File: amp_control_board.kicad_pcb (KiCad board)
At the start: 2 copper layers, 75 parts, among them J1 Conn_01x03_Male, J2 Conn_01x04_Female, J3 Screw_Terminal_01x03, J4 Screw_Terminal_01x02, J5 Conn_01x04_Female, J6 Conn_02x03_Odd_Even, J7 Conn_01x03_Male, M1 Fan_4pin, M2 Fan_4pin, Q1 BSP89, Q2 BSP89, Q3 BSS138, Q4 BSS138, SW1 SW_Push, SW2 SW_Push, SW3 SW_Push, SW4 SW_Push, U1 L7805, U2 L7812, U3 LD1117V33-DG, U4 MCP4251-xxxx-SL, U5 STM32F103C8Tx, Y1 8M, Y2 32.768

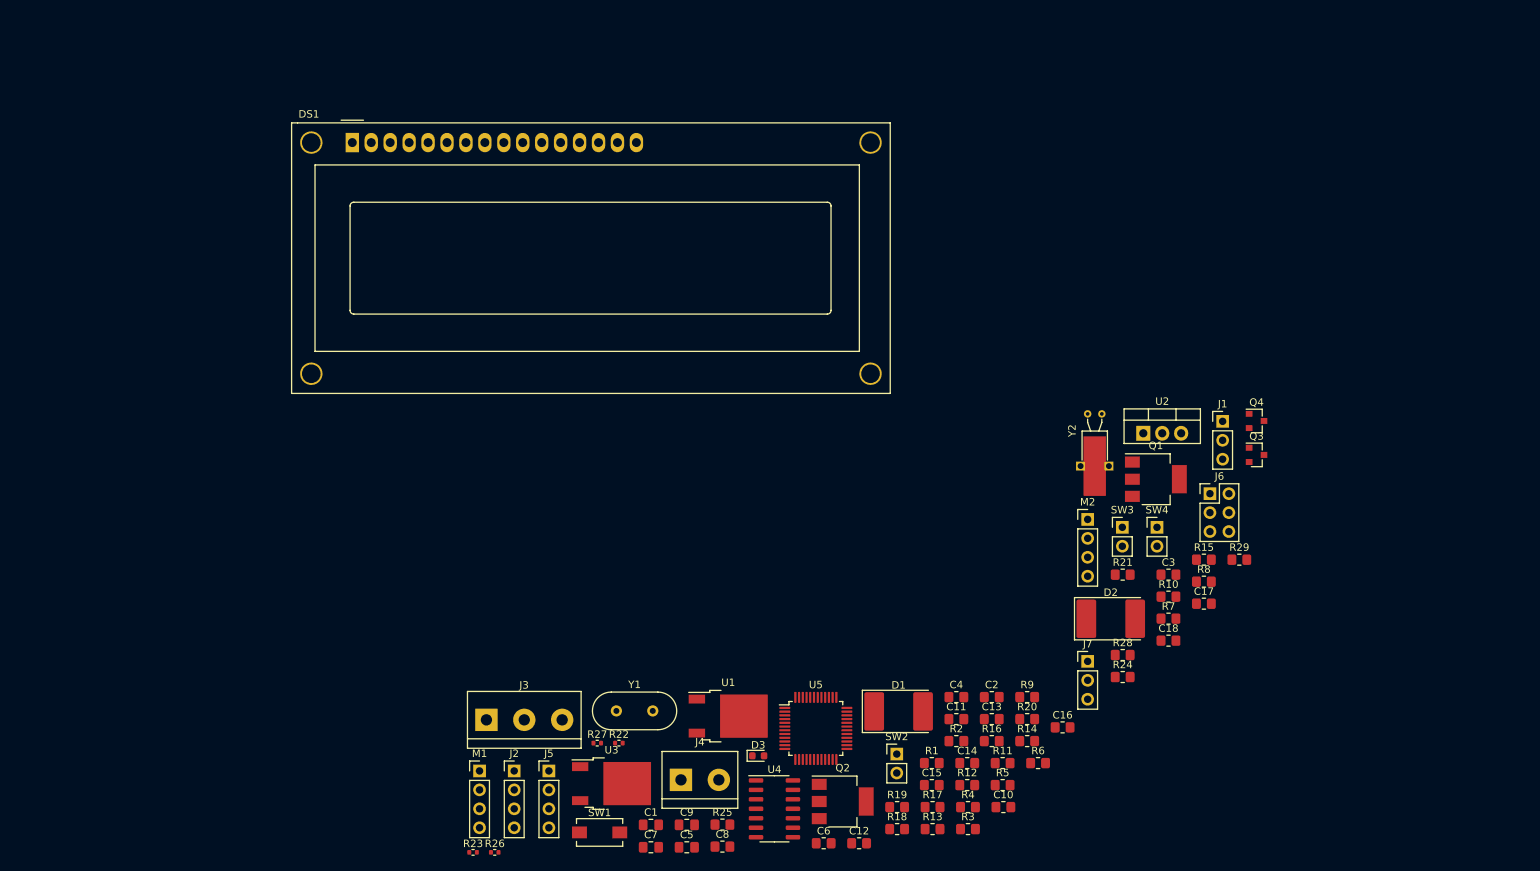
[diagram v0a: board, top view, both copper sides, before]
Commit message: changing dev pc
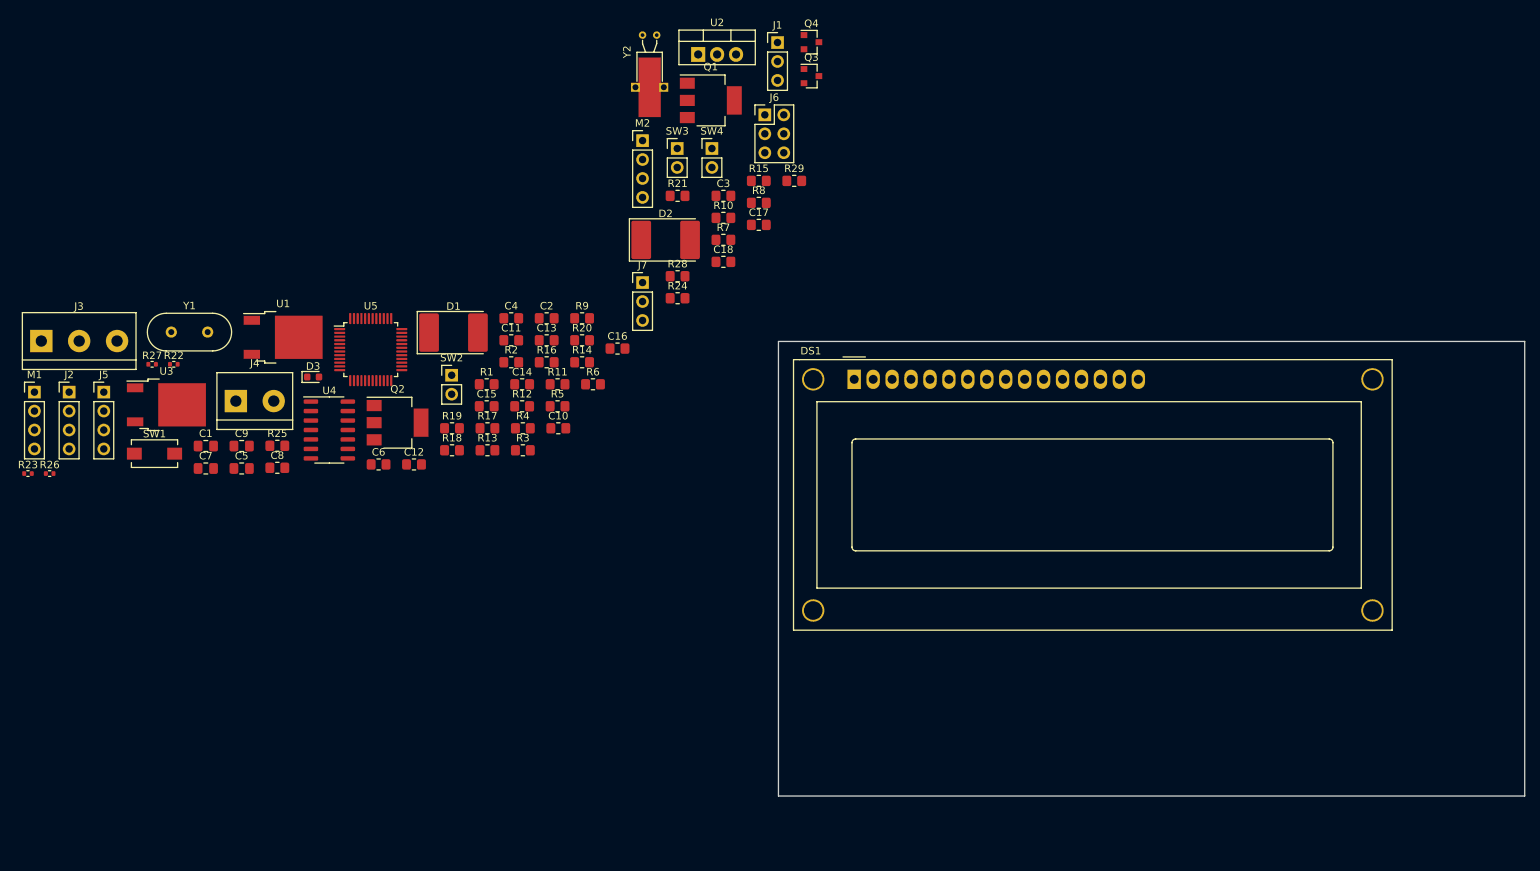
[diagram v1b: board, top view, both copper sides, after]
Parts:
- moved SW3 78.4 mm to (113.4, 40.2)
- moved SW4 78.4 mm to (118.1, 40.2)
- moved U3 78.4 mm to (44.9, 74.5)
- moved C10 78.4 mm to (97.5, 77.7)
- moved C12 78.4 mm to (78.1, 82.5)
- moved C14 78.4 mm to (92.6, 71.8)
- moved C18 78.4 mm to (119.6, 55.4)
- moved C6 78.4 mm to (73.4, 82.5)
- moved C9 78.4 mm to (55.0, 80.1)
- moved D1 78.4 mm to (83.4, 64.9)
- moved D2 78.4 mm to (111.9, 52.4)
- moved J3 78.4 mm to (28.1, 66.0)
- moved J4 78.4 mm to (54.2, 74.0)
- moved J6 78.4 mm to (125.2, 35.7)
- moved J7 78.4 mm to (108.8, 58.1)
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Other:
- board outline added: 100.1 x 61 mm
- rule trace_min: 0.2 -> 0.1016
- rule via_min_drill: 0.3 -> 0.254
- rule via_min_size: 0.4 -> 0.254
